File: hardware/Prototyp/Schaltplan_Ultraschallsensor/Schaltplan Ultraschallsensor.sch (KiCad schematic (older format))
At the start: 21 parts, among them IC1 A5950, P1 CON-SENSOR2, P2 CONN_01X05, U1 XMC1XXX40, X1 CRYSTAL_3225

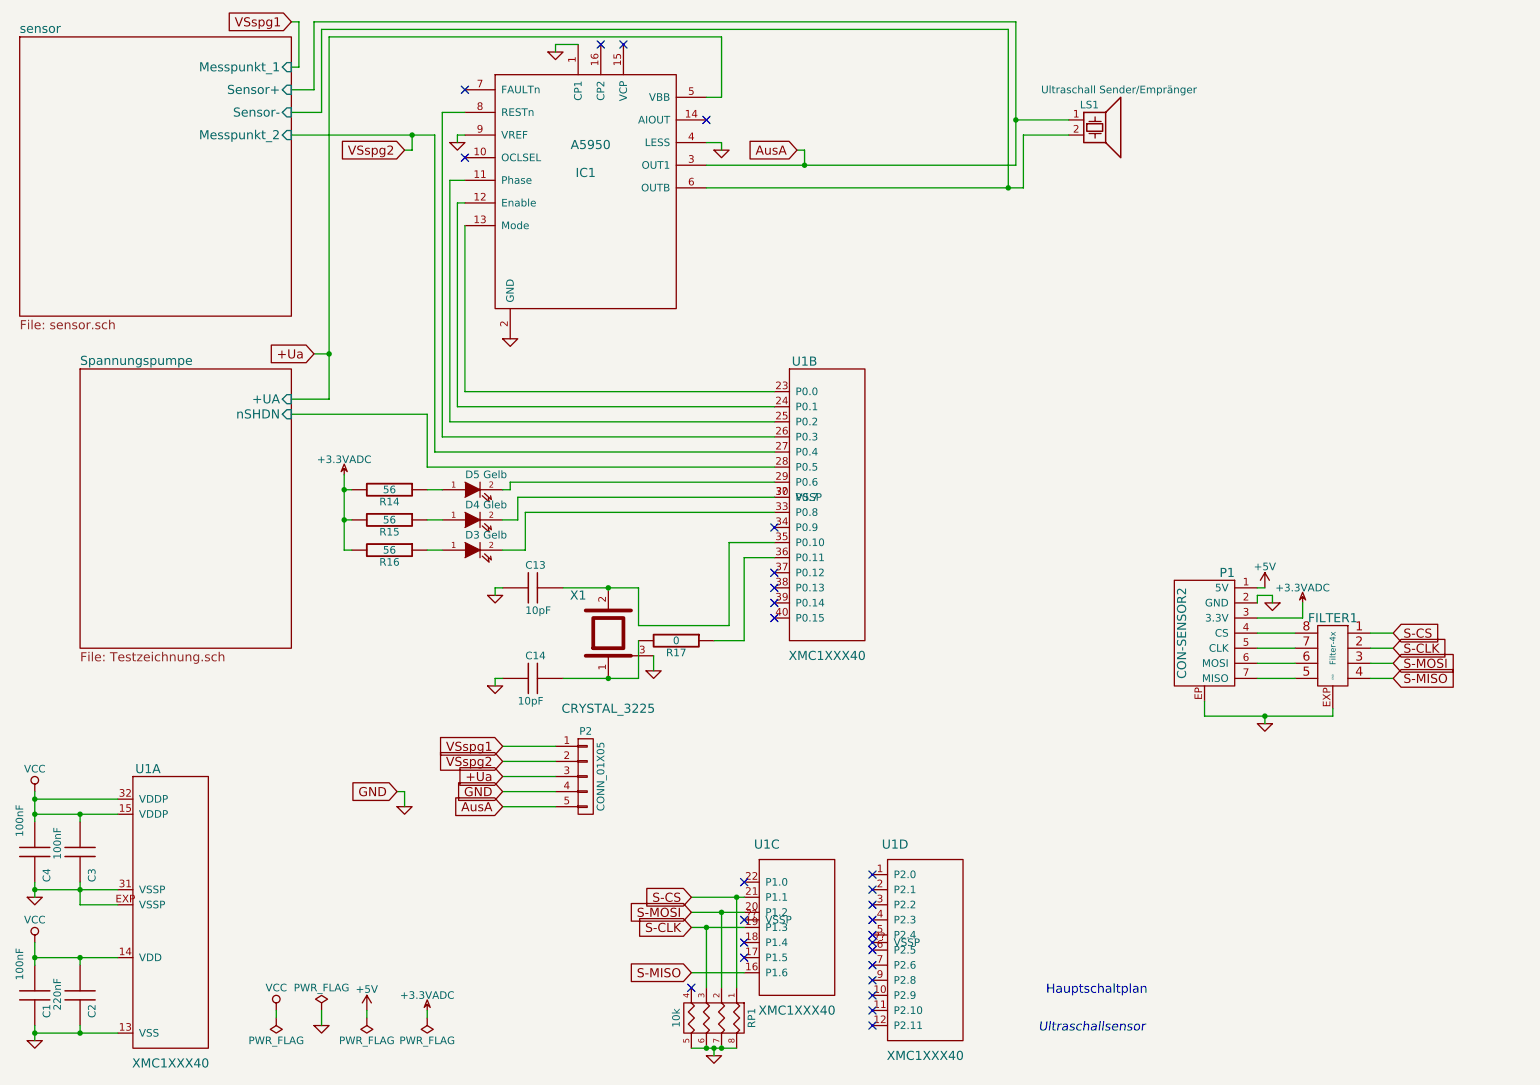
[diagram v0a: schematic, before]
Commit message: Platinenlayout
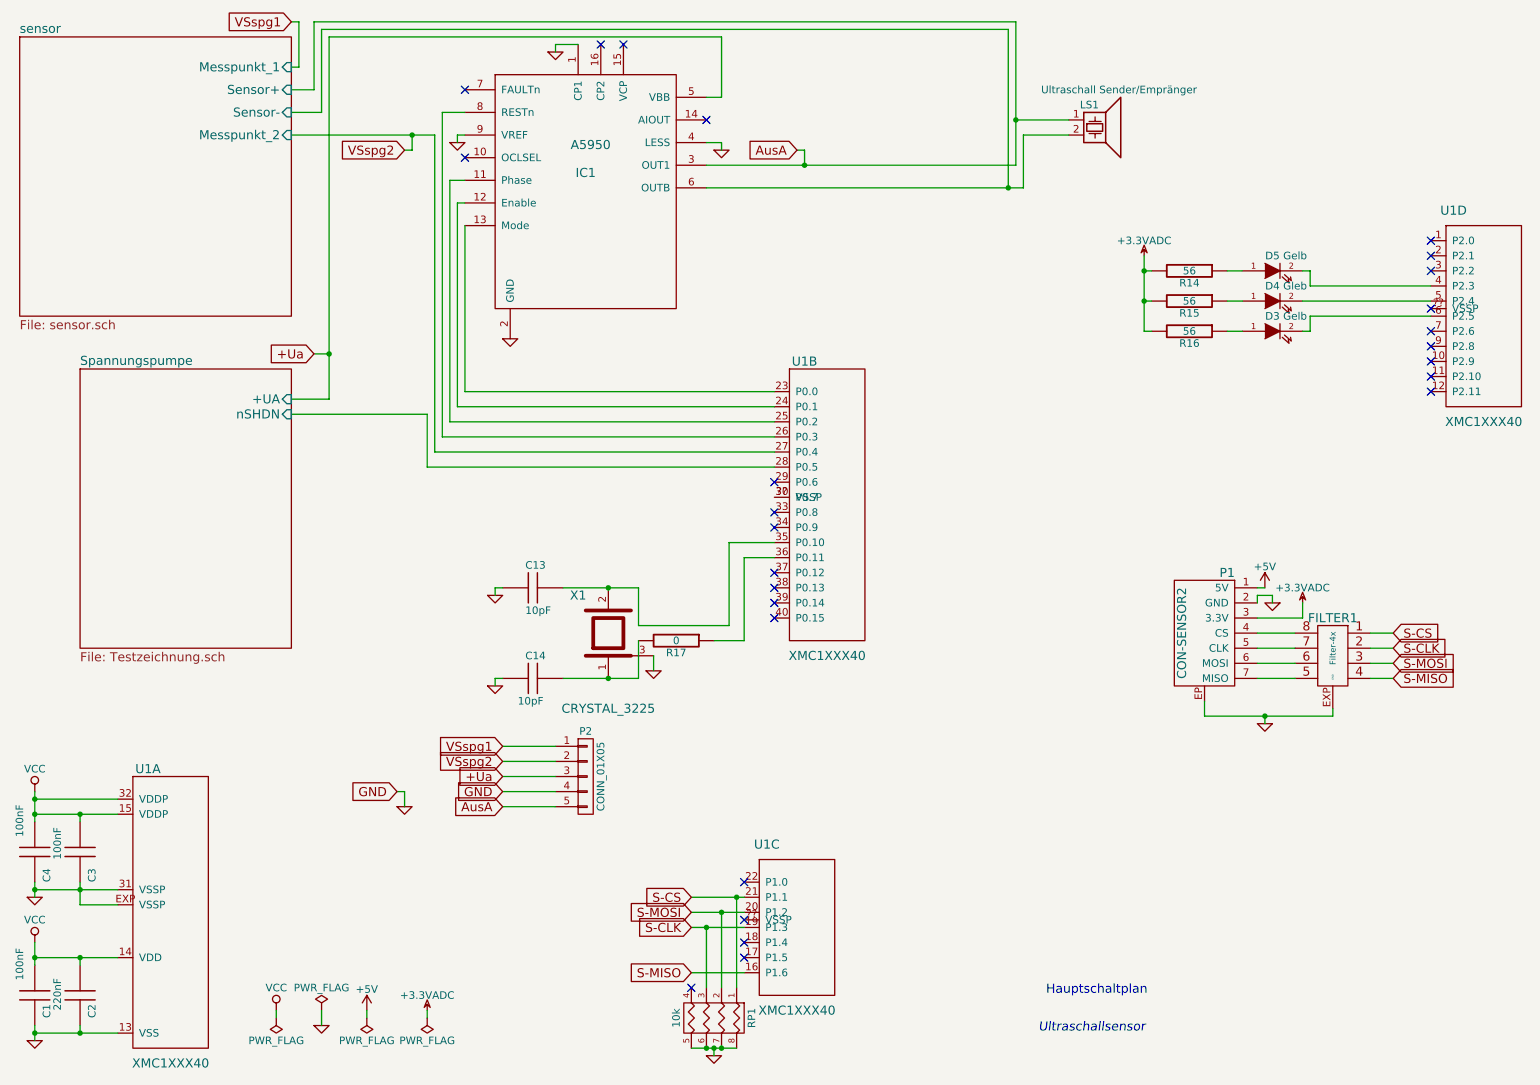
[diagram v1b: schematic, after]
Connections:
- net at U1.29 (P0.6): no longer D5.2 (K)
- net at U1.30 (P0.7), U1.?? (VSSP): no longer D4.2 (K)
- net at U1.33 (P0.8): no longer D3.2 (K)
- net at U1.4 (P2.3): now also D5.2 (K)
- net at U1.5 (P2.4): now also D4.2 (K)
- net at U1.6 (P2.5): now also D3.2 (K)
- no-connect marks 27 -> 26
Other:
- moved on the sheet: D3, D4, D5, R14, R15, R16, U1D
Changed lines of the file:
@@
 L XMC1XXX40 U1
 U 4 1 5A70A99D
-P 6600 6950
-F 0 "U1" H 6400 7650 60  0000 C CNN
-F 1 "XMC1XXX40" H 6600 6250 60  0000 C CNN
-F 2 "kicad-libraries:HVQFN40-6x6" H 6750 7700 60  0001 C CNN
-F 3 "" H 6750 7700 60  0000 C CNN
-	4    6600 6950
+P 10300 2750
+F 0 "U1" H 10100 3450 60  0000 C CNN
+F 1 "XMC1XXX40" H 10300 2050 60  0000 C CNN
+F 2 "kicad-libraries:HVQFN40-6x6" H 10450 3500 60  0001 C CNN
+F 3 "" H 10450 3500 60  0000 C CNN
+	4    10300 2750
 	1    0    0    -1
 $EndComp
@@
 	3450 1850 3450 3450
 Connection ~ 7150 1900
-NoConn ~ 6250 7450
-NoConn ~ 6250 7350
-NoConn ~ 6250 7250
-NoConn ~ 6250 7150
-NoConn ~ 6250 7050
-NoConn ~ 6250 6950
-NoConn ~ 6250 6900
-NoConn ~ 6250 6850
-NoConn ~ 6250 6750
-NoConn ~ 6250 6650
-NoConn ~ 6250 6550
-NoConn ~ 6250 6450
+NoConn ~ 9950 3250
+NoConn ~ 9950 3150
+NoConn ~ 9950 3050
+NoConn ~ 9950 2950
+NoConn ~ 9950 2850
+NoConn ~ 9950 2700
+NoConn ~ 9950 2450
+NoConn ~ 9950 2350
+NoConn ~ 9950 2250
 NoConn ~ 5400 7000
 NoConn ~ 5400 6900
@@
 L LED D5
 U 1 1 5A7323BC
-P 3600 3900
-F 0 "D5" H 3600 4000 50  0000 C CNN
-F 1 "Gelb" H 3750 4000 50  0000 C CNN
-F 2 "kicad-libraries:D0603E" H 3600 3900 50  0001 C CNN
-F 3 "" H 3600 3900 50  0000 C CNN
-	1    3600 3900
+P 8900 2450
+F 0 "D5" H 8900 2550 50  0000 C CNN
+F 1 "Gelb" H 9050 2550 50  0000 C CNN
+F 2 "kicad-libraries:D0603E" H 8900 2450 50  0001 C CNN
+F 3 "" H 8900 2450 50  0000 C CNN
+	1    8900 2450
 	1    0    0    -1
 $EndComp
@@
 L LED D4
 U 1 1 5A732455
-P 3600 4100
-F 0 "D4" H 3600 4200 50  0000 C CNN
-F 1 "Gleb" H 3750 4200 50  0000 C CNN
-F 2 "kicad-libraries:D0603E" H 3600 4100 50  0001 C CNN
-F 3 "" H 3600 4100 50  0000 C CNN
-	1    3600 4100
+P 8900 2650
+F 0 "D4" H 8900 2750 50  0000 C CNN
+F 1 "Gleb" H 9050 2750 50  0000 C CNN
+F 2 "kicad-libraries:D0603E" H 8900 2650 50  0001 C CNN
+F 3 "" H 8900 2650 50  0000 C CNN
+	1    8900 2650
 	1    0    0    -1
 $EndComp
@@
 L LED D3
 U 1 1 5A7324B4
-P 3600 4300
-F 0 "D3" H 3600 4400 50  0000 C CNN
-F 1 "Gelb" H 3750 4400 50  0000 C CNN
-F 2 "kicad-libraries:D0603E" H 3600 4300 50  0001 C CNN
-F 3 "" H 3600 4300 50  0000 C CNN
-	1    3600 4300
-	1    0    0    -1
-$EndComp
-Wire Wire Line
-	2750 3800 2750 4300
-Wire Wire Line
-	2750 4100 2800 4100
-Connection ~ 2750 3900
-Wire Wire Line
-	2750 4300 2800 4300
-Connection ~ 2750 4100
-Wire Wire Line
-	2800 3900 2750 3900
+P 8900 2850
+F 0 "D3" H 8900 2950 50  0000 C CNN
+F 1 "Gelb" H 9050 2950 50  0000 C CNN
+F 2 "kicad-libraries:D0603E" H 8900 2850 50  0001 C CNN
+F 3 "" H 8900 2850 50  0000 C CNN
+	1    8900 2850
+	1    0    0    -1
+$EndComp
+Wire Wire Line
+	8050 2350 8050 2850
+Wire Wire Line
+	8050 2650 8100 2650
+Connection ~ 8050 2450
+Wire Wire Line
+	8050 2850 8100 2850
+Connection ~ 8050 2650
+Wire Wire Line
+	8100 2450 8050 2450
 $Comp
 L R R14
 U 1 1 5A74243E
-P 3050 3900
-F 0 "R14" V 3130 3900 50  0000 C CNN
-F 1 "56" V 3050 3900 50  0000 C CNN
-F 2 "kicad-libraries:R0603F" H 3050 3900 60  0001 C CNN
-F 3 "" H 3050 3900 60  0000 C CNN
-	1    3050 3900
+P 8350 2450
+F 0 "R14" V 8430 2450 50  0000 C CNN
+F 1 "56" V 8350 2450 50  0000 C CNN
+F 2 "kicad-libraries:R0603F" H 8350 2450 60  0001 C CNN
+F 3 "" H 8350 2450 60  0000 C CNN
+	1    8350 2450
 	0    1    1    0
 $EndComp
@@
 L R R15
 U 1 1 5A742BF8
-P 3050 4100
-F 0 "R15" V 3130 4100 50  0000 C CNN
-F 1 "56" V 3050 4100 50  0000 C CNN
-F 2 "kicad-libraries:R0603F" H 3050 4100 60  0001 C CNN
-F 3 "" H 3050 4100 60  0000 C CNN
-	1    3050 4100
+P 8350 2650
+F 0 "R15" V 8430 2650 50  0000 C CNN
+F 1 "56" V 8350 2650 50  0000 C CNN
+F 2 "kicad-libraries:R0603F" H 8350 2650 60  0001 C CNN
+F 3 "" H 8350 2650 60  0000 C CNN
+	1    8350 2650
 	0    1    1    0
 $EndComp
@@
 L R R16
 U 1 1 5A742C8A
-P 3050 4300
-F 0 "R16" V 3130 4300 50  0000 C CNN
-F 1 "56" V 3050 4300 50  0000 C CNN
-F 2 "kicad-libraries:R0603F" H 3050 4300 60  0001 C CNN
-F 3 "" H 3050 4300 60  0000 C CNN
-	1    3050 4300
+P 8350 2850
+F 0 "R16" V 8430 2850 50  0000 C CNN
+F 1 "56" V 8350 2850 50  0000 C CNN
+F 2 "kicad-libraries:R0603F" H 8350 2850 60  0001 C CNN
+F 3 "" H 8350 2850 60  0000 C CNN
+	1    8350 2850
 	0    1    1    0
 $EndComp
 Wire Wire Line
-	3300 3900 3400 3900
-Wire Wire Line
-	3400 4100 3300 4100
-Wire Wire Line
-	3300 4300 3400 4300
+	8600 2450 8700 2450
+Wire Wire Line
+	8700 2650 8600 2650
+Wire Wire Line
+	8600 2850 8700 2850
 $Comp
 L +3.3VADC #PWR019
@@
 L +3.3VADC #PWR021
 U 1 1 5A744D41
-P 2750 3800
-F 0 "#PWR021" H 2900 3750 50  0001 C CNN
-F 1 "+3.3VADC" H 2750 3900 50  0000 C CNN
-F 2 "" H 2750 3800 50  0001 C CNN
-F 3 "" H 2750 3800 50  0001 C CNN
-	1    2750 3800
+P 8050 2350
+F 0 "#PWR021" H 8200 2300 50  0001 C CNN
+F 1 "+3.3VADC" H 8050 2450 50  0000 C CNN
+F 2 "" H 8050 2350 50  0001 C CNN
+F 3 "" H 8050 2350 50  0001 C CNN
+	1    8050 2350
 	1    0    0    -1
 $EndComp
@@
 	5300 4250 5600 4250
 Wire Wire Line
-	3800 3900 3850 3900
-Wire Wire Line
-	3850 3900 3850 3850
-Wire Wire Line
-	3850 3850 5600 3850
-Wire Wire Line
-	3800 4100 3900 4100
-Wire Wire Line
-	3900 4100 3900 3950
-Wire Wire Line
-	3900 3950 5600 3950
-Wire Wire Line
-	3800 4300 3950 4300
-Wire Wire Line
-	3950 4300 3950 4050
-Wire Wire Line
-	3950 4050 5600 4050
+	9100 2450 9150 2450
+Wire Wire Line
+	9100 2650 9950 2650
 NoConn ~ 5600 4150
 NoConn ~ 5600 4450
@@
 	5050 7100 5400 7100
 NoConn ~ 5050 7200
+NoConn ~ 5600 3850
+NoConn ~ 5600 4050
+Wire Wire Line
+	9950 2550 9150 2550
+Wire Wire Line
+	9150 2550 9150 2450
+Wire Wire Line
+	9100 2850 9150 2850
+Wire Wire Line
+	9150 2850 9150 2750
+Wire Wire Line
+	9150 2750 9950 2750
 $EndSCHEMATC
